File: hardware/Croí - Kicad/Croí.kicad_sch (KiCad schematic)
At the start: 5 parts, among them J1 2060-1452/998-404, J2 ESQ-110-X-X-D, U1 NUP2105LT1G, U2 STM32F411CEUx

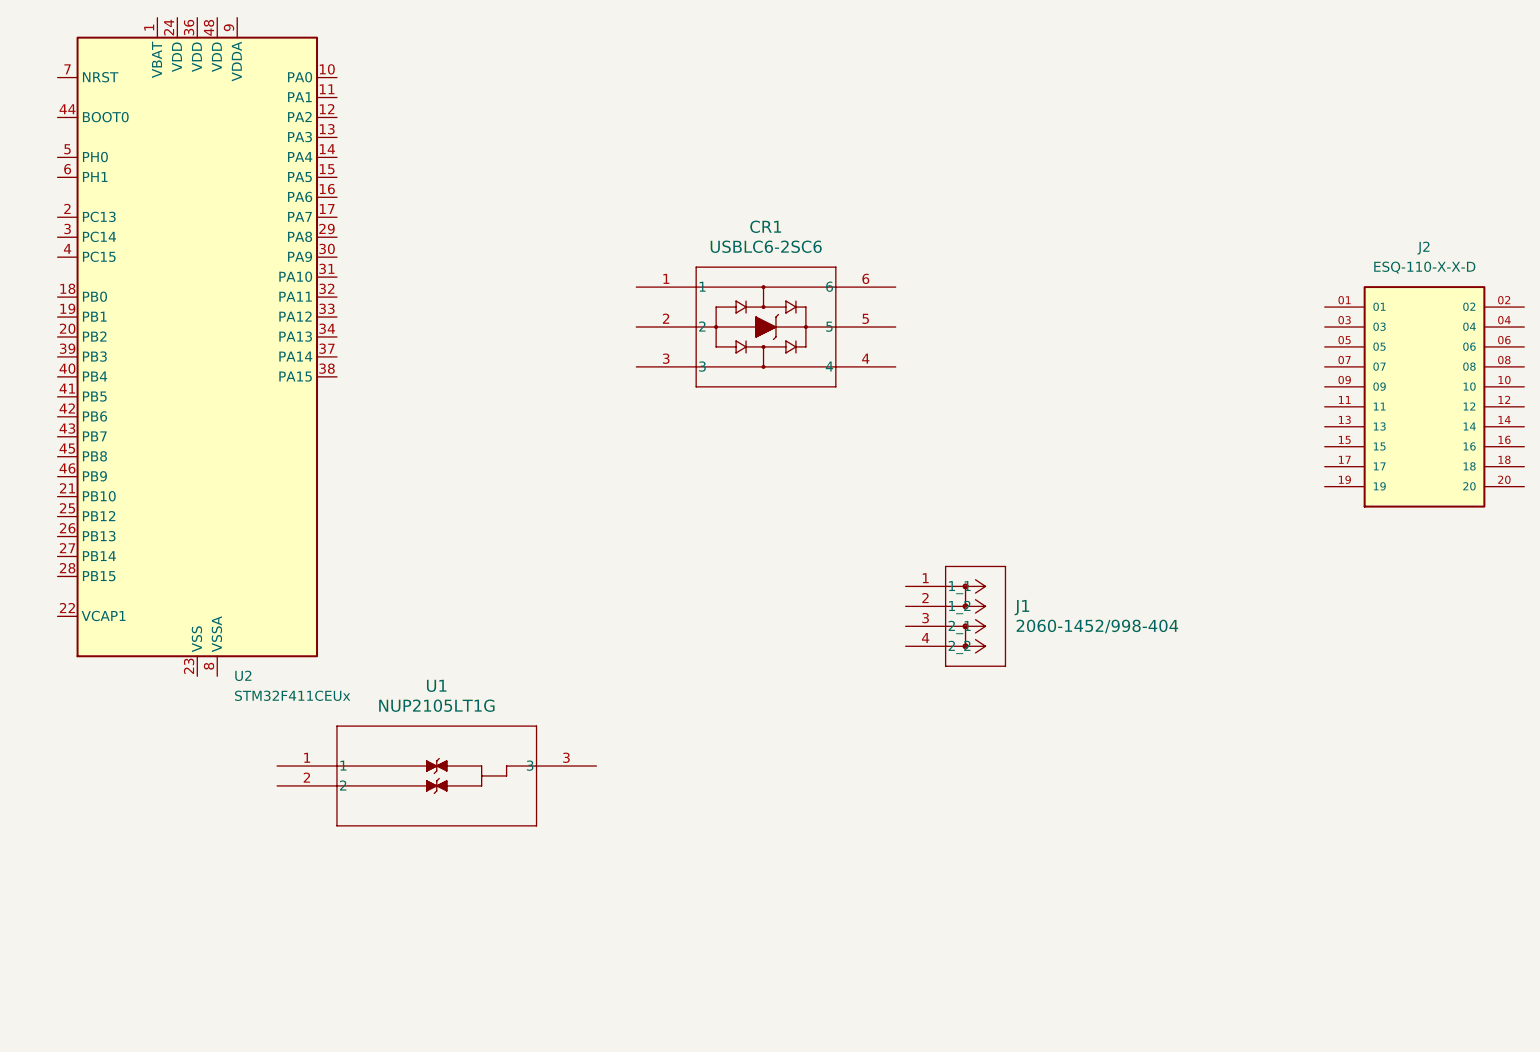
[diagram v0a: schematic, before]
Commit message: minor junctions
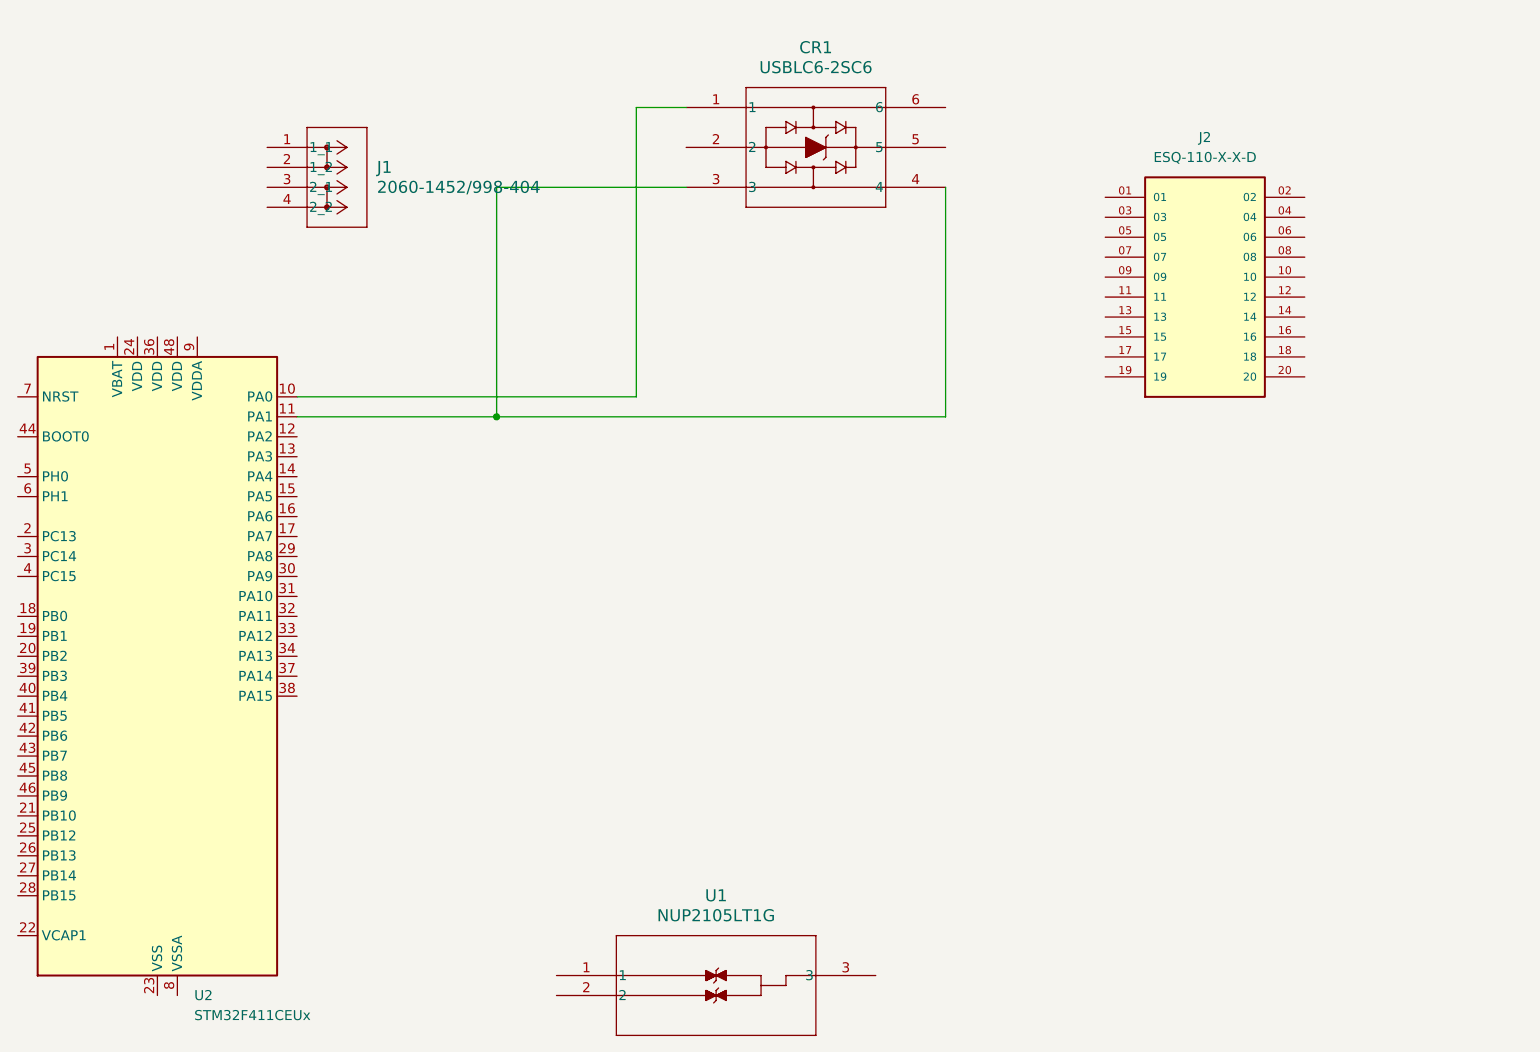
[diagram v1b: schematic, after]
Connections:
- net at U2.10 (PA0): now also CR1.1
- net at U2.11 (PA1): now also CR1.3, CR1.4
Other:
- moved on the sheet: CR1, J1, J2, U1, U2
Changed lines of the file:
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@@
 	(generator_version "9.0")
 	(paper "A4")
+	(junction
+		(at 93.98 64.77)
+		(diameter 0)
+		(color 0 0 0 0)
+	)
+	(wire
+		(pts
+			(xy 151.13 64.77) (xy 93.98 64.77)
+		)
+		(stroke
+			(width 0)
+			(type default)
+		)
+	)
+	(wire
+		(pts
+			(xy 118.11 25.4) (xy 111.76 25.4)
+		)
+		(stroke
+			(width 0)
+			(type default)
+		)
+	)
+	(wire
+		(pts
+			(xy 93.98 64.77) (xy 68.58 64.77)
+		)
+		(stroke
+			(width 0)
+			(type default)
+		)
+	)
+	(wire
+		(pts
+			(xy 111.76 25.4) (xy 111.76 62.23)
+		)
+		(stroke
+			(width 0)
+			(type default)
+		)
+	)
+	(wire
+		(pts
+			(xy 93.98 35.56) (xy 93.98 64.77)
+		)
+		(stroke
+			(width 0)
+			(type default)
+		)
+	)
+	(wire
+		(pts
+			(xy 111.76 62.23) (xy 68.58 62.23)
+		)
+		(stroke
+			(width 0)
+			(type default)
+		)
+	)
+	(wire
+		(pts
+			(xy 151.13 35.56) (xy 151.13 64.77)
+		)
+		(stroke
+			(width 0)
+			(type default)
+		)
+	)
+	(wire
+		(pts
+			(xy 118.11 35.56) (xy 93.98 35.56)
+		)
+		(stroke
+			(width 0)
+			(type default)
+		)
+	)
 	(symbol
 		(lib_id "ESQ:ESQ-110-X-X-D")
-		(at 212.09 60.96 0)
+		(at 184.15 46.99 0)
 		(unit 1)
 		(exclude_from_sim no)
@@
 		(fields_autoplaced yes)
 		(property "Reference" "J2"
-			(at 212.09 43.18 0)
+			(at 184.15 29.21 0)
 			(effects
 				(font
@@
 		)
 		(property "Value" "ESQ-110-X-X-D"
-			(at 212.09 45.72 0)
+			(at 184.15 31.75 0)
 			(effects
 				(font
@@
 		)
 		(property "Footprint" "SAMTEC_ESQ-110-14-G-D"
-			(at 212.09 60.96 0)
+			(at 184.15 46.99 0)
 			(effects
 				(font
@@
 		)
 		(property "Datasheet" ""
-			(at 212.09 60.96 0)
+			(at 184.15 46.99 0)
 			(effects
 				(font
@@
 		)
 		(property "Description" ""
-			(at 212.09 60.96 0)
+			(at 184.15 46.99 0)
 			(effects
 				(font
@@
 		)
 		(property "MF" "Samtec"
-			(at 212.09 60.96 0)
+			(at 184.15 46.99 0)
 			(effects
 				(font
@@
 		)
 		(property "Description_1" "20 Position Elevated Socket Connector 0.100 (2.54mm) Through Hole Gold"
-			(at 212.09 60.96 0)
+			(at 184.15 46.99 0)
 			(effects
 				(font
@@
 		)
 		(property "Package" "None"
-			(at 212.09 60.96 0)
+			(at 184.15 46.99 0)
 			(effects
 				(font
@@
 		)
 		(property "Price" "None"
-			(at 212.09 60.96 0)
+			(at 184.15 46.99 0)
 			(effects
 				(font
@@
 		)
 		(property "Check_prices" "https://www.snapeda.com/parts/ESQ-110-14-G-D-LL/Samtec/view-part/?ref=eda"
-			(at 212.09 60.96 0)
+			(at 184.15 46.99 0)
 			(effects
 				(font
@@
 		)
 		(property "STANDARD" "Manufacturer Recommendations"
-			(at 212.09 60.96 0)
+			(at 184.15 46.99 0)
 			(effects
 				(font
@@
 		)
 		(property "PARTREV" "NA"
-			(at 212.09 60.96 0)
+			(at 184.15 46.99 0)
 			(effects
 				(font
@@
 		)
 		(property "SnapEDA_Link" "https://www.snapeda.com/parts/ESQ-110-14-G-D-LL/Samtec/view-part/?ref=snap"
-			(at 212.09 60.96 0)
+			(at 184.15 46.99 0)
 			(effects
 				(font
@@
 		)
 		(property "MP" "ESQ-110-14-G-D-LL"
-			(at 212.09 60.96 0)
+			(at 184.15 46.99 0)
 			(effects
 				(font
@@
 		)
 		(property "Purchase-URL" "https://www.snapeda.com/api/url_track_click_mouser/?unipart_id=3563488&manufacturer=Samtec&part_name=ESQ-110-14-G-D-LL&search_term=esq-110-14-g-d-ll"
-			(at 212.09 60.96 0)
+			(at 184.15 46.99 0)
 			(effects
 				(font
@@
 		)
 		(property "Availability" "In Stock"
-			(at 212.09 60.96 0)
+			(at 184.15 46.99 0)
 			(effects
 				(font
@@
 		)
 		(property "MANUFACTURER" "Samtec"
-			(at 212.09 60.96 0)
+			(at 184.15 46.99 0)
 			(effects
 				(font
@@
 	(symbol
 		(lib_id "1:NUP2105LT1G")
-		(at 66.04 109.22 0)
+		(at 101.6 135.89 0)
 		(unit 1)
 		(exclude_from_sim no)
@@
 		(fields_autoplaced yes)
 		(property "Reference" "U1"
-			(at 86.36 99.06 0)
+			(at 121.92 125.73 0)
 			(effects
 				(font
@@
 		)
 		(property "Value" "NUP2105LT1G"
-			(at 86.36 101.6 0)
+			(at 121.92 128.27 0)
 			(effects
 				(font
@@
 		)
 		(property "Footprint" "SOT-23_3L_ONS"
-			(at 66.04 109.22 0)
+			(at 101.6 135.89 0)
 			(effects
 				(font
@@
 		)
 		(property "Datasheet" "NUP2105LT1G"
-			(at 66.04 109.22 0)
+			(at 101.6 135.89 0)
 			(effects
 				(font
@@
 		)
 		(property "Description" ""
-			(at 66.04 109.22 0)
+			(at 101.6 135.89 0)
 			(effects
 				(font
@@
 	(symbol
 		(lib_id "MCU_ST_STM32F4:STM32F411CEUx")
-		(at 55.88 57.15 0)
+		(at 50.8 97.79 0)
 		(unit 1)
 		(exclude_from_sim no)
@@
 		(fields_autoplaced yes)
 		(property "Reference" "U2"
-			(at 60.5633 97.79 0)
+			(at 55.4833 138.43 0)
 			(effects
 				(font
@@
 		)
 		(property "Value" "STM32F411CEUx"
-			(at 60.5633 100.33 0)
+			(at 55.4833 140.97 0)
 			(effects
 				(font
@@
 		)
 		(property "Footprint" "Package_DFN_QFN:QFN-48-1EP_7x7mm_P0.5mm_EP5.6x5.6mm"
-			(at 40.64 95.25 0)
+			(at 35.56 135.89 0)
 			(effects
 				(font
@@
 		)
 		(property "Datasheet" "https://www.st.com/resource/en/datasheet/stm32f411ce.pdf"
-			(at 55.88 57.15 0)
+			(at 50.8 97.79 0)
 			(effects
 				(font
@@
 		)
 		(property "Description" "STMicroelectronics Arm Cortex-M4 MCU, 512KB flash, 128KB RAM, 100 MHz, 1.7-3.6V, 36 GPIO, UFQFPN48"
-			(at 55.88 57.15 0)
+			(at 50.8 97.79 0)
 			(effects
 				(font
@@
 	(symbol
 		(lib_id "usb:USBLC6-2SC6")
-		(at 111.76 48.26 0)
+		(at 118.11 25.4 0)
 		(unit 1)
 		(exclude_from_sim no)
@@
 		(fields_autoplaced yes)
 		(property "Reference" "CR1"
-			(at 128.27 40.64 0)
+			(at 134.62 17.78 0)
 			(effects
 				(font
@@
 		)
 		(property "Value" "USBLC6-2SC6"
-			(at 128.27 43.18 0)
+			(at 134.62 20.32 0)
 			(effects
 				(font
@@
 		)
 		(property "Footprint" "SOT23-6L_STM"
-			(at 111.76 48.26 0)
+			(at 118.11 25.4 0)
 			(effects
 				(font
@@
 		)
 		(property "Datasheet" "https://www.st.com/resource/en/datasheet/usblc6-2.pdf"
-			(at 111.76 48.26 0)
+			(at 118.11 25.4 0)
 			(effects
 				(font
@@
 		)
 		(property "Description" ""
-			(at 111.76 48.26 0)
+			(at 118.11 25.4 0)
 			(effects
 				(font
@@
 	(symbol
 		(lib_id "wago:2060-1452_998-404")
-		(at 146.05 86.36 0)
+		(at 64.77 30.48 0)
 		(unit 1)
 		(exclude_from_sim no)
@@
 		(fields_autoplaced yes)
 		(property "Reference" "J1"
-			(at 160.02 88.8999 0)
+			(at 78.74 33.0199 0)
 			(effects
 				(font
@@
 		)
 		(property "Value" "2060-1452/998-404"
-			(at 160.02 91.4399 0)
+			(at 78.74 35.5599 0)
 			(effects
 				(font
@@
 		)
 		(property "Footprint" "WAG"
-			(at 146.05 86.36 0)
+			(at 64.77 30.48 0)
 			(effects
 				(font
@@
 		)
 		(property "Datasheet" "2060-1452/998-404"
-			(at 146.05 86.36 0)
+			(at 64.77 30.48 0)
 			(effects
 				(font
@@
 		)
 		(property "Description" ""
-			(at 146.05 86.36 0)
-			(effects
-				(font
+			(at 64.77 30.48 0)
+			(effects
+				(font
